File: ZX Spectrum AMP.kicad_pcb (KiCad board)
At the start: 2 copper layers, 55 x 48 mm, 13 parts, among them IC1 LM386, J1 9V DC(in), J2 Input (MIC), J3 9V DC(out), P1 4,7K Ohm

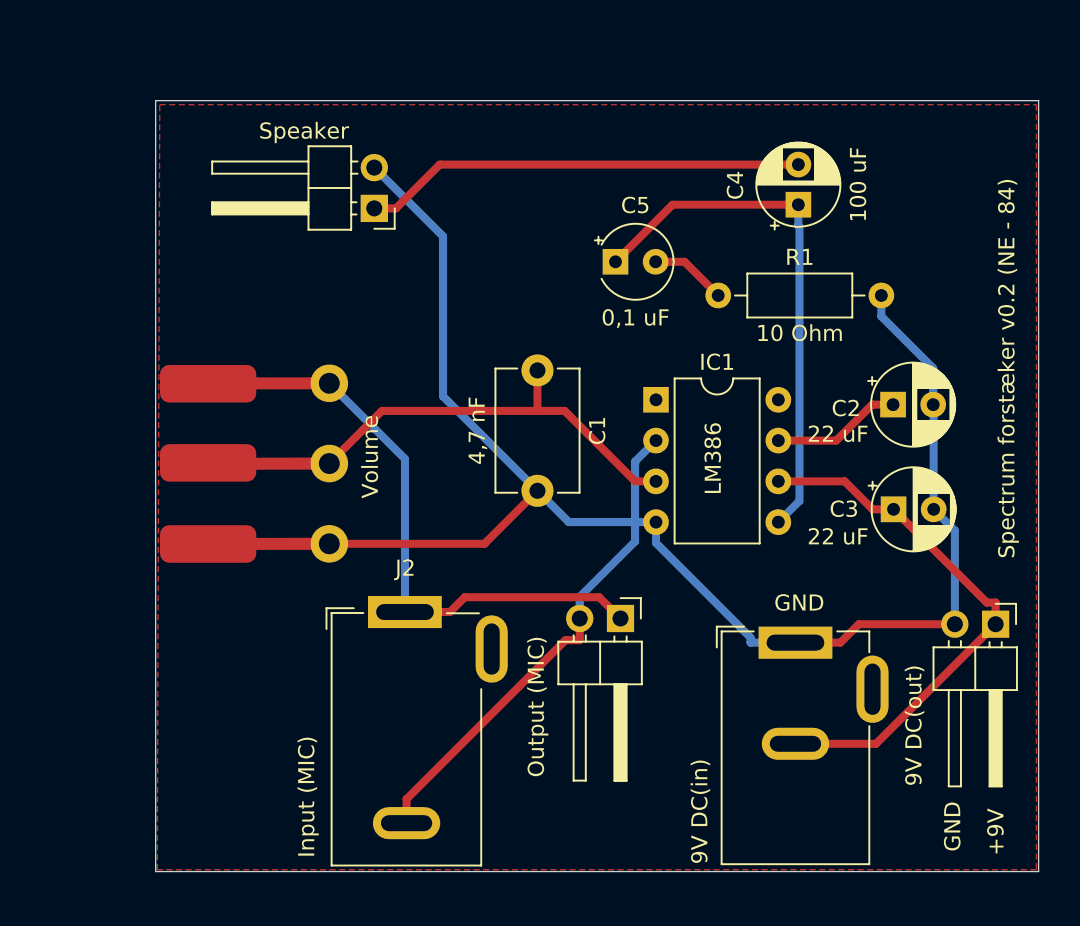
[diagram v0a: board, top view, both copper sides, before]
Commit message: updated
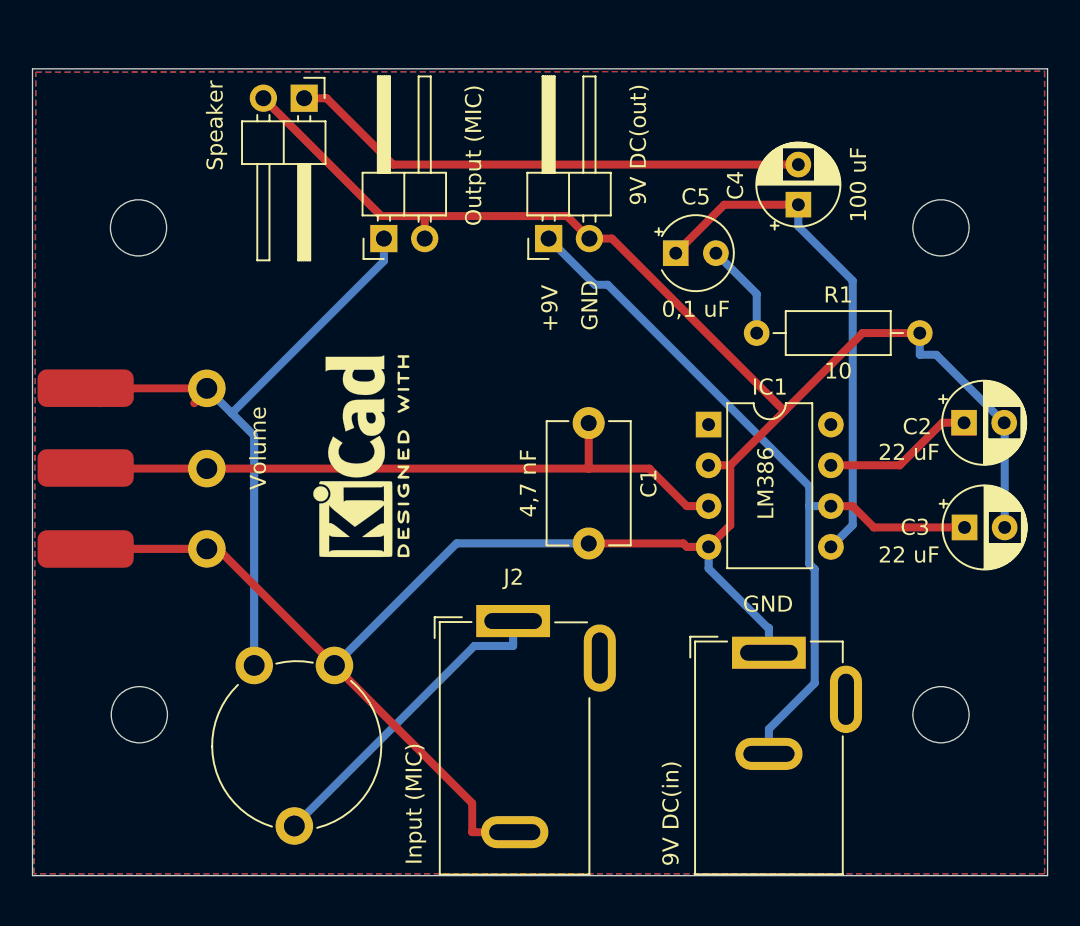
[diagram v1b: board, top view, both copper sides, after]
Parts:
- added G***: LOGO, LOGO, F.Cu at (59.5, 59.9)
- added H1: MountingHole, MountingHole:MountingHole_3.5mm, F.Cu at (34.5, 44.8)
- added H2: MountingHole, MountingHole:MountingHole_3.5mm, F.Cu at (84.5, 44.8)
- added H3: MountingHole, MountingHole:MountingHole_3.5mm, F.Cu at (34.5, 75.1)
- added H4: MountingHole, MountingHole:MountingHole_3.5mm, F.Cu at (84.5, 75.1)
- added P2: 50K, Potentiometer_THT:Potentiometer_Piher_PT-10-V10_Vertical, F.Cu at (41.7, 72.0)
- added REF**: KiCad-Logo2_5mm_SilkScreen, Symbol:KiCad-Logo2_5mm_SilkScreen, F.Cu at (48.4, 59.0)
- P1: value 4,7K Ohm -> 4.7K
- R1: value 10 Ohm -> 10
- moved J3 36.8 mm to (60.0, 45.4), turned to 90 degrees
- moved MIC1 27.9 mm to (49.8, 45.4), turned to 90 degrees
- moved HT1 8.14 mm to (44.8, 36.7), turned to -90 degrees
- moved P1 7.63 mm to (38.8, 54.7)
- moved J2 6.76 mm to (57.9, 69.2)
- moved C1 4.57 mm to (62.5, 56.9)
- moved C2 4.56 mm to (85.9, 56.9)
- moved C3 4.56 mm to (85.9, 63.4)
- moved C5 3.79 mm to (68.0, 46.3)
- moved IC1 3.62 mm to (70.0, 57.0)
- moved R1 3.35 mm to (73.0, 51.3)
- moved J1 1.77 mm to (73.8, 71.2)
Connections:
- J2 pad 1: Net-(MIC1-Pin_1) -> Net-(J2-Pad1)
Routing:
- net Net-(J2-Pad1): track 0.00 -> 19.8 mm
- net GND: track 130.7 -> 148.9 mm
- net +9V: track 33.6 -> 50.8 mm
- net Net-(IC1-+): track 33.6 -> 42.6 mm
- net Net-(MIC1-Pin_1): track 38.1 -> 43.4 mm
- net Net-(C4-Pad2): track 27.5 -> 32.5 mm
- net Net-(IC1-BYPASS): track 8.07 -> 9.39 mm
- net Net-(C5-Pad2): track 4.77 -> 6.03 mm
- net Net-(C4-Pad1): track 33.2 -> 32.2 mm
- added copper zone on B.Cu, net GND
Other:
- board size 55 x 48 mm -> 63.2 x 50.3 mm
